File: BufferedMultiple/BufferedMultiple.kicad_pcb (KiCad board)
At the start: 2 copper layers, 20.3 x 128.5 mm, 18 parts

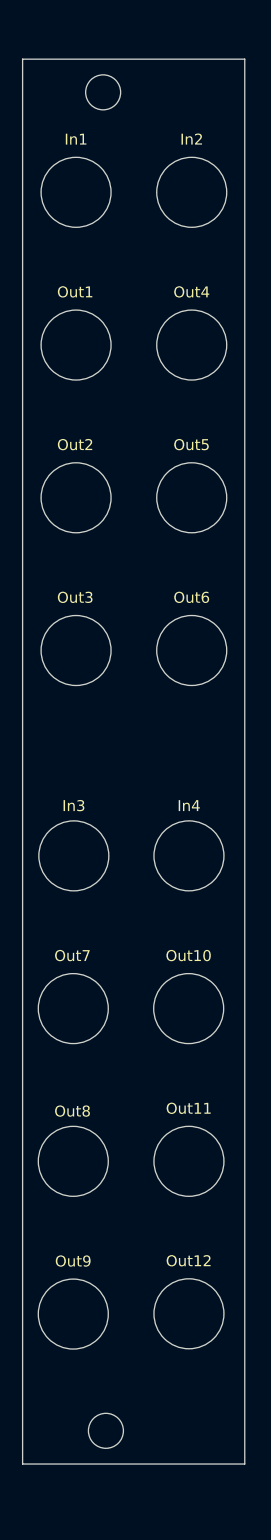
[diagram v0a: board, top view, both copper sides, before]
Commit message: WIP: faceplate design
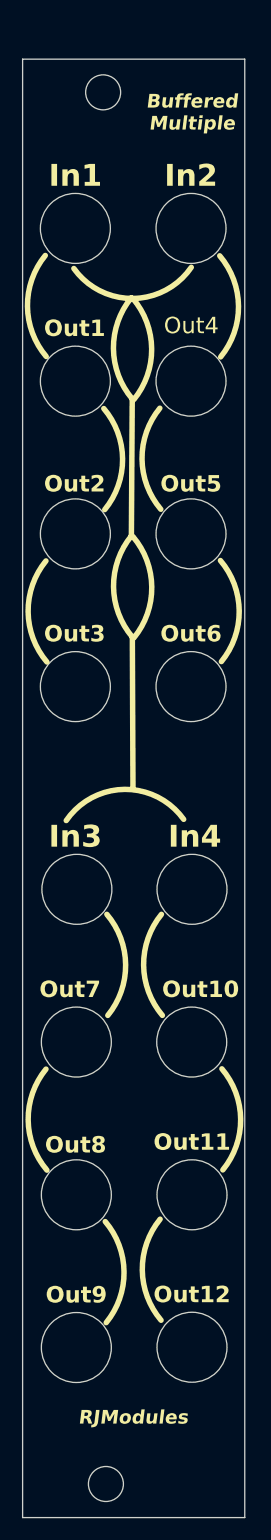
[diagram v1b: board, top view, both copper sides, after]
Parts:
- moved fbmhb 4.86 mm to (160.0, 163.9)
- moved Out2 3.30 mm to (157.2, 77.0)
- moved Out3 3.30 mm to (157.2, 90.9)
- moved Out5 3.30 mm to (167.8, 77.0)
- moved Out6 3.30 mm to (167.8, 90.9)
- moved In1 3.30 mm to (157.2, 49.0)
- moved In2 3.30 mm to (167.8, 49.0)
- moved Out1 3.30 mm to (157.2, 63.0)
- moved Out4 3.30 mm to (167.8, 63.0)
- moved In4 3.07 mm to (167.9, 109.5)
- moved Out12 3.07 mm to (167.9, 151.4)
- moved Out7 3.07 mm to (157.3, 123.4)
- moved In3 3.07 mm to (157.4, 109.5)
- moved Out10 3.07 mm to (167.9, 123.4)
- moved Out11 3.07 mm to (167.9, 137.4)
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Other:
- board size 20.3 x 128.5 mm -> 20.3 x 133.4 mm
- board text added: "Buffered Multiple"
- board text added: "RJModules"

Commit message: sent to production v1.0.0
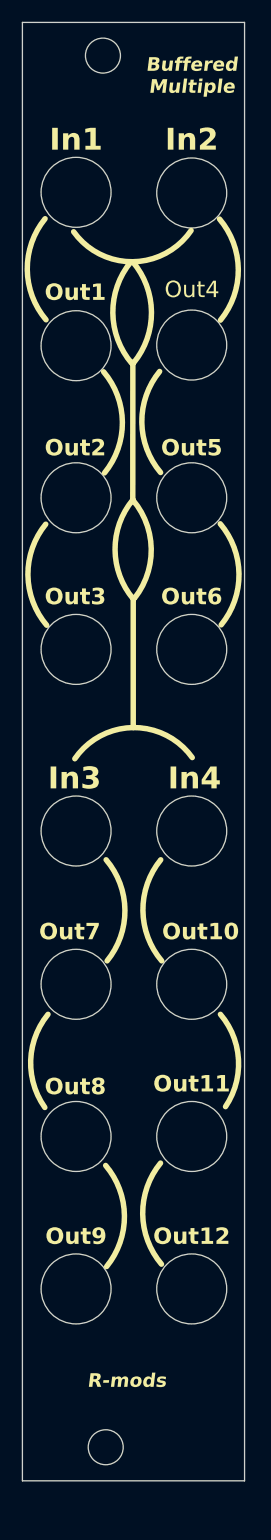
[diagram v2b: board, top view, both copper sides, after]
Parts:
- moved Out9 5.36 mm to (157.3, 146.0)
- moved In3 5.33 mm to (157.3, 104.1)
- moved In4 5.33 mm to (167.9, 104.1)
- moved Out12 5.33 mm to (167.9, 146.0)
- moved Out11 5.33 mm to (167.9, 132.1)
- moved Out8 5.33 mm to (157.3, 132.1)
- moved Out7 5.28 mm to (157.3, 118.2)
- moved Out10 5.28 mm to (167.9, 118.2)
- moved Out3 3.40 mm to (157.3, 87.5)
- moved Out6 3.40 mm to (167.9, 87.5)
- moved fbmhb 3.36 mm to (160.0, 160.5)
- moved fpmht 3.36 mm to (159.7, 33.2)
- moved Out2 3.30 mm to (157.3, 73.7)
- moved Out5 3.30 mm to (167.9, 73.7)
- moved In1 3.30 mm to (157.3, 45.7)
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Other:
- board text added: "R-mods"
- board text removed: "RJModules"
